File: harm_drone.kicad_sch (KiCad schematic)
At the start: 13 parts, among them IC1 Microcontroller, J1 SYS_DEBUG

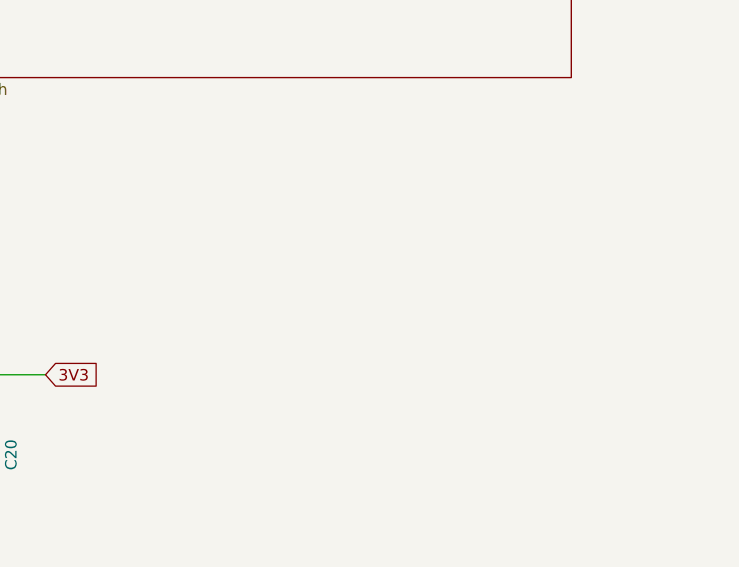
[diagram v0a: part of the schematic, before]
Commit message: before model updates
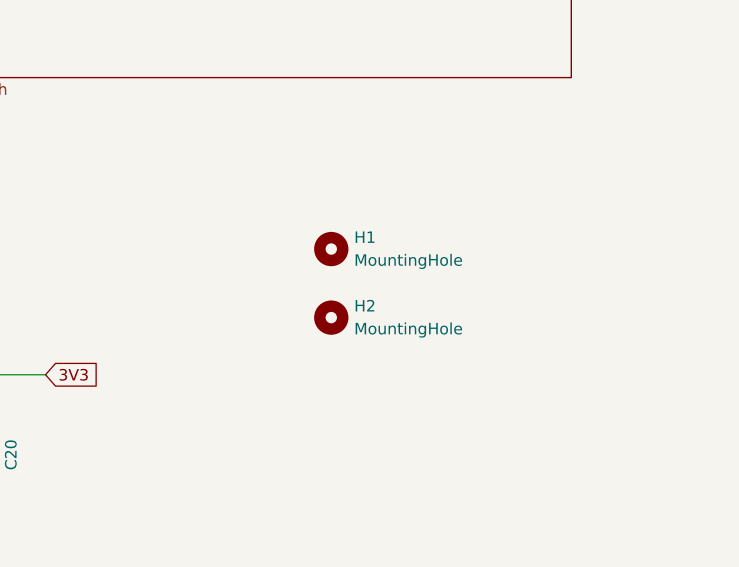
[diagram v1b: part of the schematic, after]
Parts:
- added H1, H2: MountingHole, MountingHole:MountingHole_3.2mm_M3, symbol Mechanical:MountingHole
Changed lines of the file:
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@@
+	)
+	(symbol
+		(lib_id "Mechanical:MountingHole")
+		(at 240.03 83.82 0)
+		(unit 1)
+		(exclude_from_sim yes)
+		(in_bom no)
+		(on_board yes)
+		(dnp no)
+		(fields_autoplaced yes)
+		(property "Reference" "H1"
+			(at 242.57 82.5499 0)
+			(effects
+				(font
+					(size 1.27 1.27)
+				)
+				(justify left)
+			)
+		)
+		(property "Value" "MountingHole"
+			(at 242.57 85.0899 0)
+			(effects
+				(font
+					(size 1.27 1.27)
+				)
+				(justify left)
+			)
+		)
+		(property "Footprint" "MountingHole:MountingHole_3.2mm_M3"
+			(at 240.03 83.82 0)
+			(effects
+				(font
+					(size 1.27 1.27)
+				)
+				(hide yes)
+			)
+		)
+		(property "Datasheet" "~"
+			(at 240.03 83.82 0)
+			(effects
+				(font
+					(size 1.27 1.27)
+				)
+				(hide yes)
+			)
+		)
+		(property "Description" "Mounting Hole without connection"
+			(at 240.03 83.82 0)
+			(effects
+				(font
+					(size 1.27 1.27)
+				)
+				(hide yes)
+			)
+		)
+		(instances
+			(project ""
+				(path "/5ce3566e-4e0f-420e-9b0d-3952cd3c63fd"
+					(reference "H1")
+					(unit 1)
+				)
+			)
+		)
 	)
 	(symbol
@@
 					(unit 1)
 				)
+			)
+		)
+	)
+	(symbol
+		(lib_id "Mechanical:MountingHole")
+		(at 240.03 91.44 0)
+		(unit 1)
+		(exclude_from_sim yes)
+		(in_bom no)
+		(on_board yes)
+		(dnp no)
+		(fields_autoplaced yes)
+		(property "Reference" "H2"
+			(at 242.57 90.1699 0)
+			(effects
+				(font
+					(size 1.27 1.27)
+				)
+				(justify left)
+			)
+		)
+		(property "Value" "MountingHole"
+			(at 242.57 92.7099 0)
+			(effects
+				(font
+					(size 1.27 1.27)
+				)
+				(justify left)
+			)
+		)
+		(property "Footprint" "MountingHole:MountingHole_3.2mm_M3"
+			(at 240.03 91.44 0)
+			(effects
+				(font
+					(size 1.27 1.27)
+				)
+				(hide yes)
+			)
+		)
+		(property "Datasheet" "~"
+			(at 240.03 91.44 0)
+			(effects
+				(font
+					(size 1.27 1.27)
+				)
+				(hide yes)
+			)
+		)
+		(property "Description" "Mounting Hole without connection"
+			(at 240.03 91.44 0)
+			(effects
+				(font
+					(size 1.27 1.27)
+				)
+				(hide yes)
+			)
+		)
+		(instances
+			(project "harm_drone"
+				(path "/5ce3566e-4e0f-420e-9b0d-3952cd3c63fd"
+					(reference "H2")
+					(unit 1)
+				)

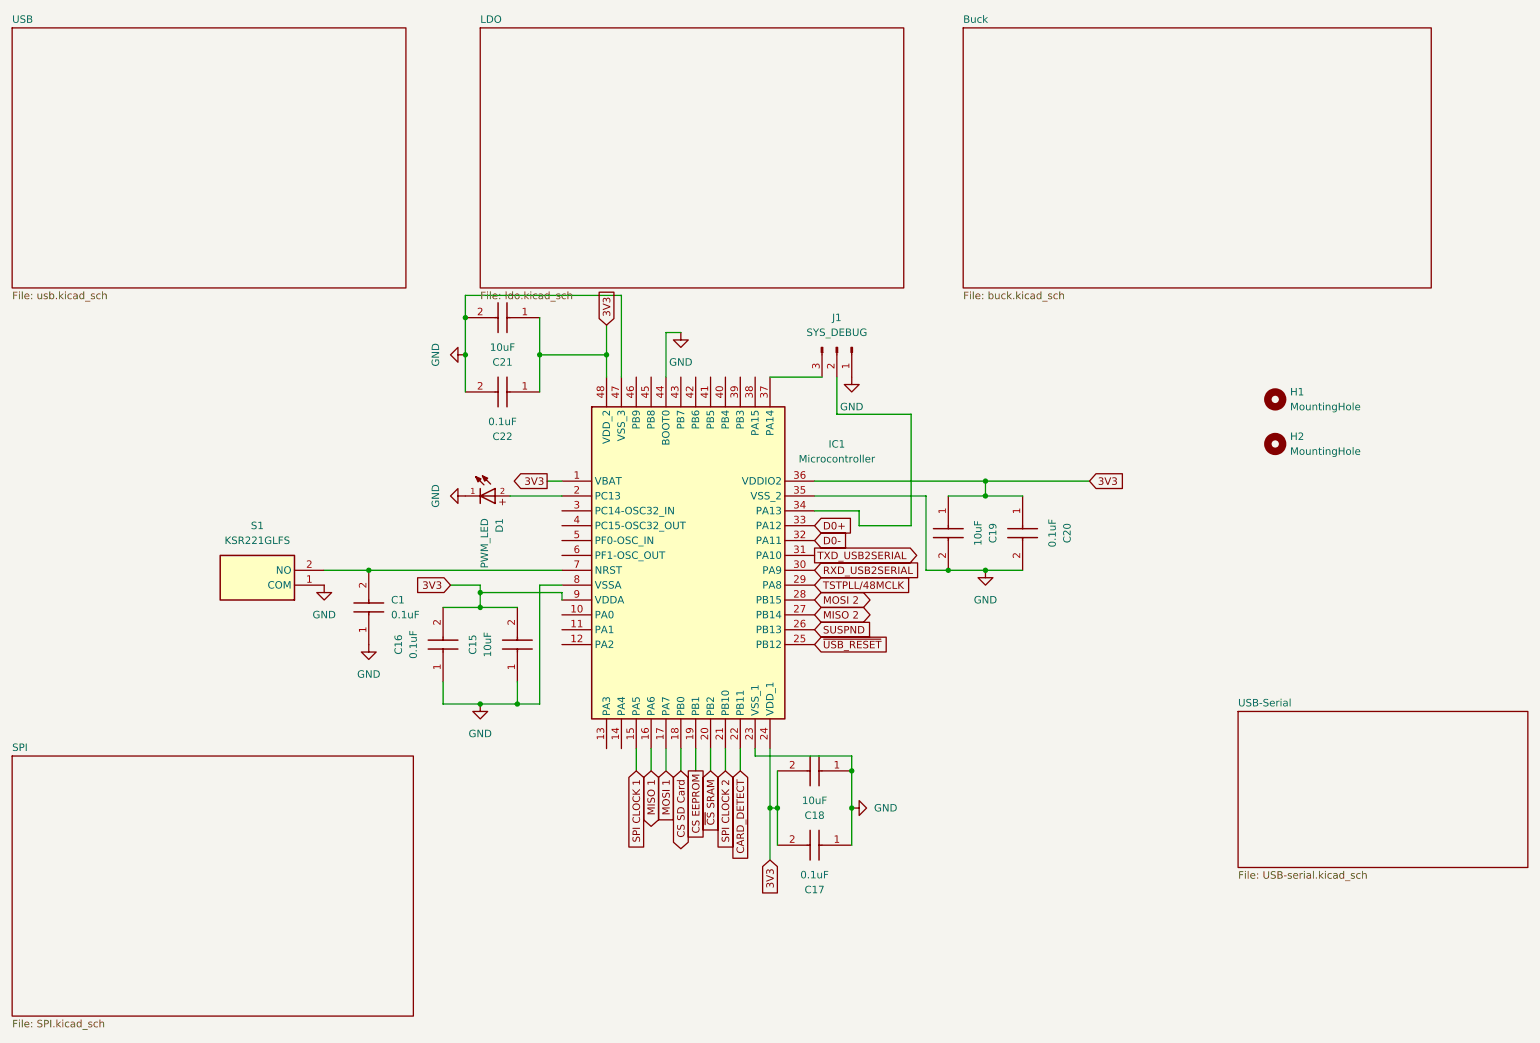
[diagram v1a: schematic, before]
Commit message: schematic fixes are done
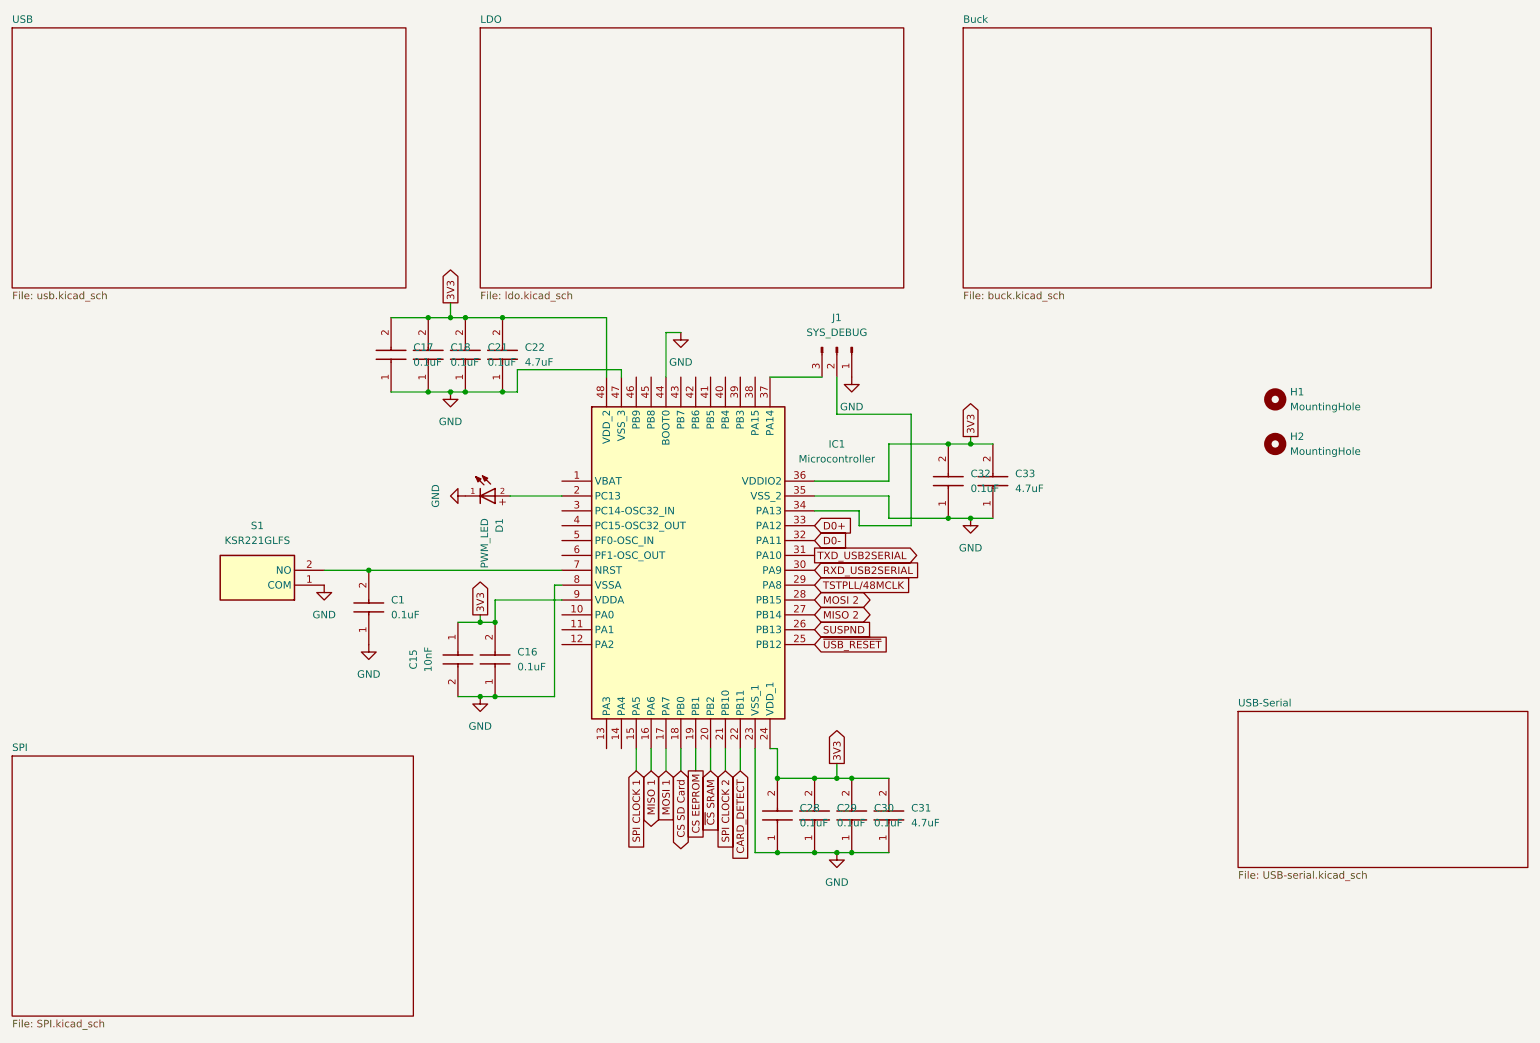
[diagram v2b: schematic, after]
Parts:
- removed C19: 10uF, Capacitor_SMD:C_0805_2012Metric, symbol group127:0805Capacitor
- removed C20: 0.1uF, Capacitor_SMD:C_0805_2012Metric, symbol group127:0805Capacitor
- added C28, C29, C30, C32: 0.1uF, Capacitor_SMD:C_0805_2012Metric, symbol group127:0805Capacitor
- added C31, C33: 4.7uF, Capacitor_SMD:C_0805_2012Metric, symbol group127:0805Capacitor
- C15: value 10uF -> 10nF
- C18, C21: value 10uF -> 0.1uF
- C22: value 0.1uF -> 4.7uF
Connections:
- net 3V3: now also C15.1, C21.2, C22.2, C28.2, C29.2, C30.2, C31.2, C32.2, C33.2; no longer C15.2, C21.1, C22.1, IC1.1 (VBAT)
- net GND: now also C15.2, C21.1, C22.1, C28.1, C29.1, C30.1, C31.1, C32.1, C33.1; no longer C15.1, C21.2, C22.2

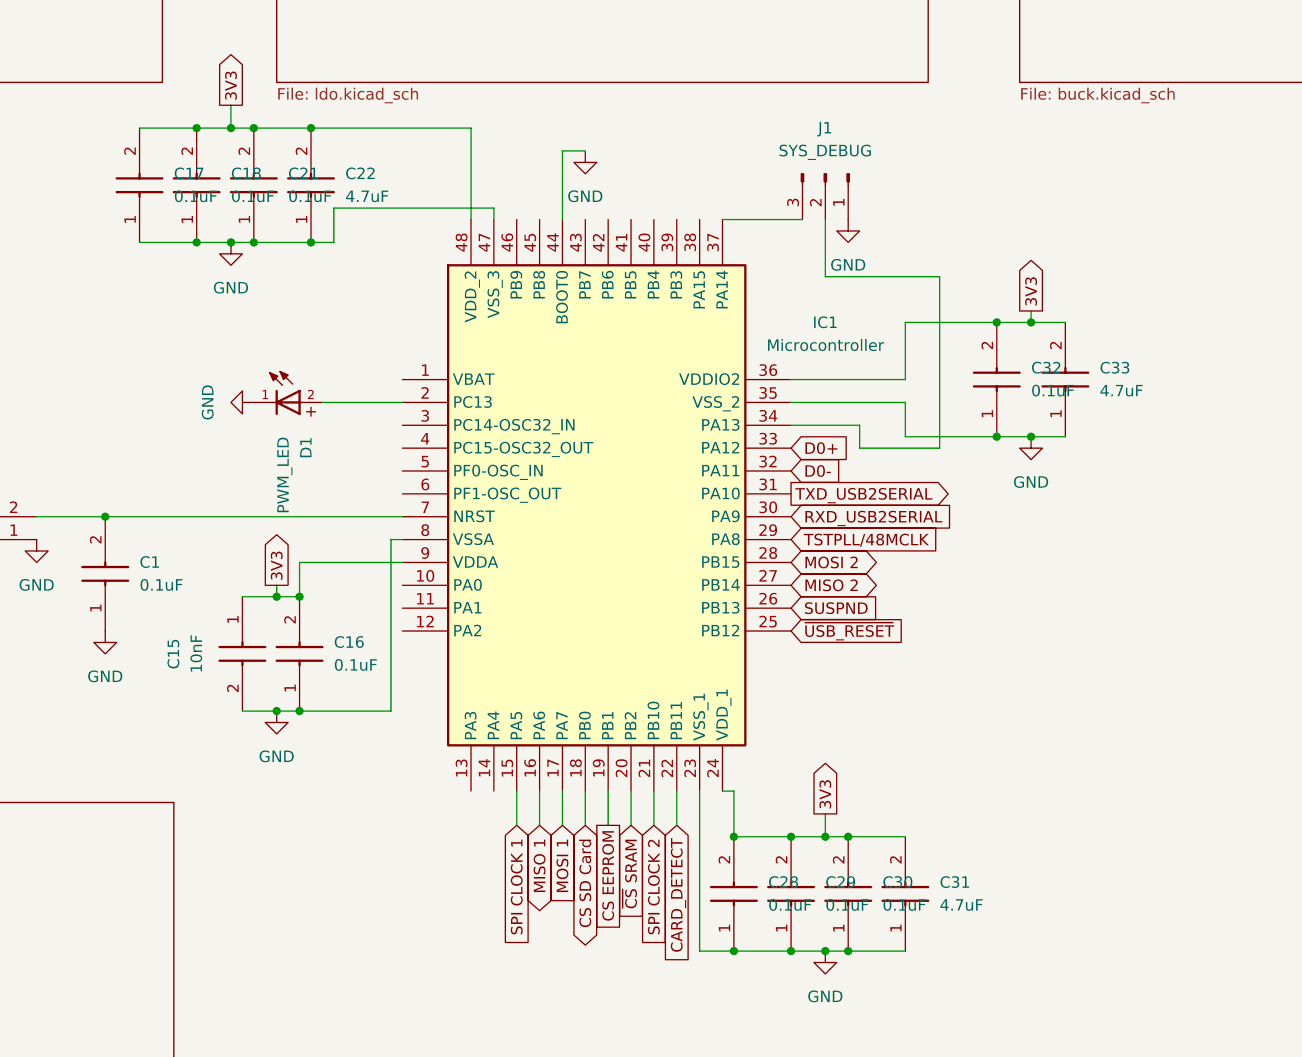
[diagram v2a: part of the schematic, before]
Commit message: final changes
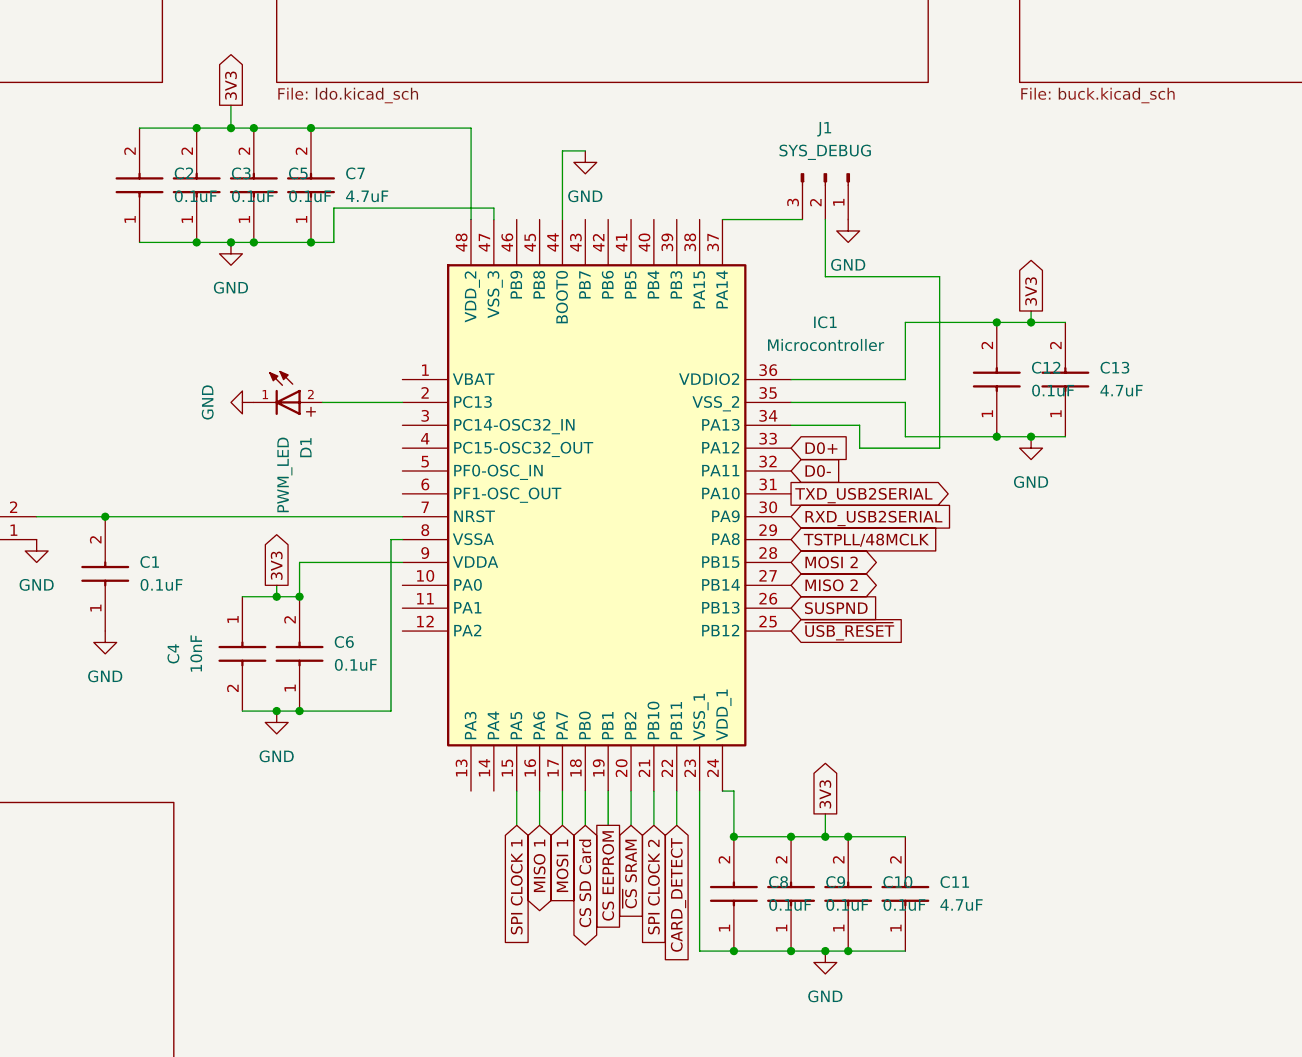
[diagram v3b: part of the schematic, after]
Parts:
- renumbered C30 to C10, C31 to C11, C32 to C12, C33 to C13, C17 to C2, C18 to C3, C15 to C4, C21 to C5, C16 to C6, C22 to C7, C28 to C8, C29 to C9
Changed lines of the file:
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@@
 		(dnp no)
 		(fields_autoplaced yes)
-		(property "Reference" "C32"
+		(property "Reference" "C12"
 			(at 187.96 96.5199 90)
 			(effects
@@
 			(project "harm_drone"
 				(path "/5ce3566e-4e0f-420e-9b0d-3952cd3c63fd"
-					(reference "C32")
+					(reference "C12")
 					(unit 1)
 				)
@@
 		(dnp no)
 		(fields_autoplaced yes)
-		(property "Reference" "C31"
+		(property "Reference" "C11"
 			(at 177.8 153.6699 90)
 			(effects
@@
 			(project "harm_drone"
 				(path "/5ce3566e-4e0f-420e-9b0d-3952cd3c63fd"
-					(reference "C31")
+					(reference "C11")
 					(unit 1)
 				)
@@
 		(dnp no)
 		(fields_autoplaced yes)
-		(property "Reference" "C33"
+		(property "Reference" "C13"
 			(at 195.58 96.5199 90)
 			(effects
@@
 			(project "harm_drone"
 				(path "/5ce3566e-4e0f-420e-9b0d-3952cd3c63fd"
-					(reference "C33")
+					(reference "C13")
 					(unit 1)
 				)
@@
 		(dnp no)
 		(fields_autoplaced yes)
-		(property "Reference" "C29"
+		(property "Reference" "C9"
 			(at 165.1 153.6699 90)
 			(effects
@@
 			(project "harm_drone"
 				(path "/5ce3566e-4e0f-420e-9b0d-3952cd3c63fd"
-					(reference "C29")
+					(reference "C9")
 					(unit 1)
 				)
@@
 		(dnp no)
 		(fields_autoplaced yes)
-		(property "Reference" "#PWR05"
+		(property "Reference" "#PWR06"
 			(at 138.43 78.74 0)
 			(effects
@@
 			(project "harm_drone"
 				(path "/5ce3566e-4e0f-420e-9b0d-3952cd3c63fd"
-					(reference "#PWR05")
+					(reference "#PWR06")
 					(unit 1)
 				)
@@
 		(dnp no)
 		(fields_autoplaced yes)
-		(property "Reference" "#PWR06"
+		(property "Reference" "#PWR05"
 			(at 104.14 140.97 0)
 			(effects
@@
 			(project "harm_drone"
 				(path "/5ce3566e-4e0f-420e-9b0d-3952cd3c63fd"
-					(reference "#PWR06")
+					(reference "#PWR05")
 					(unit 1)
 				)
@@
 		(dnp no)
 		(fields_autoplaced yes)
-		(property "Reference" "#PWR04"
+		(property "Reference" "#PWR09"
 			(at 187.96 110.49 0)
 			(effects
@@
 			(project "harm_drone"
 				(path "/5ce3566e-4e0f-420e-9b0d-3952cd3c63fd"
-					(reference "#PWR04")
+					(reference "#PWR09")
 					(unit 1)
 				)
@@
 		(dnp no)
 		(fields_autoplaced yes)
-		(property "Reference" "#PWR03"
+		(property "Reference" "#PWR07"
 			(at 165.1 167.64 0)
 			(effects
@@
 			(project "harm_drone"
 				(path "/5ce3566e-4e0f-420e-9b0d-3952cd3c63fd"
-					(reference "#PWR03")
+					(reference "#PWR07")
 					(unit 1)
 				)
@@
 		(dnp no)
 		(fields_autoplaced yes)
-		(property "Reference" "#PWR021"
+		(property "Reference" "#PWR04"
 			(at 95.25 100.33 0)
 			(effects
@@
 			(project "harm_drone"
 				(path "/5ce3566e-4e0f-420e-9b0d-3952cd3c63fd"
-					(reference "#PWR021")
+					(reference "#PWR04")
 					(unit 1)
 				)
@@
 		(dnp no)
 		(fields_autoplaced yes)
-		(property "Reference" "C18"
+		(property "Reference" "C3"
 			(at 99.06 74.9299 90)
 			(effects
@@
 			(project "harm_drone"
 				(path "/5ce3566e-4e0f-420e-9b0d-3952cd3c63fd"
-					(reference "C18")
+					(reference "C3")
 					(unit 1)
 				)
@@
 		(dnp no)
 		(fields_autoplaced yes)
-		(property "Reference" "C30"
+		(property "Reference" "C10"
 			(at 171.45 153.6699 90)
 			(effects
@@
 			(project "harm_drone"
 				(path "/5ce3566e-4e0f-420e-9b0d-3952cd3c63fd"
-					(reference "C30")
+					(reference "C10")
 					(unit 1)
 				)
@@
 		(on_board yes)
 		(dnp no)
-		(property "Reference" "C15"
+		(property "Reference" "C4"
 			(at 92.71 128.27 0)
 			(effects
@@
 			(project "harm_drone"
 				(path "/5ce3566e-4e0f-420e-9b0d-3952cd3c63fd"
-					(reference "C15")
+					(reference "C4")
 					(unit 1)
 				)
@@
 		(dnp no)
 		(fields_autoplaced yes)
-		(property "Reference" "C16"
+		(property "Reference" "C6"
 			(at 110.49 126.9999 90)
 			(effects
@@
 			(project "harm_drone"
 				(path "/5ce3566e-4e0f-420e-9b0d-3952cd3c63fd"
-					(reference "C16")
+					(reference "C6")
 					(unit 1)
 				)
@@
 		(dnp no)
 		(fields_autoplaced yes)
-		(property "Reference" "C22"
+		(property "Reference" "C7"
 			(at 111.76 74.9299 90)
 			(effects
@@
 			(project "harm_drone"
 				(path "/5ce3566e-4e0f-420e-9b0d-3952cd3c63fd"
-					(reference "C22")
+					(reference "C7")
 					(unit 1)
 				)
@@
 		(on_board yes)
 		(dnp no)
-		(property "Reference" "C28"
+		(property "Reference" "C8"
 			(at 158.75 153.6699 90)
 			(effects
@@
 			(project "harm_drone"
 				(path "/5ce3566e-4e0f-420e-9b0d-3952cd3c63fd"
-					(reference "C28")
+					(reference "C8")
 					(unit 1)
 				)
@@
 		(on_board yes)
 		(dnp no)
-		(property "Reference" "C17"
+		(property "Reference" "C2"
 			(at 92.71 74.9299 90)
 			(effects
@@
 			(project "harm_drone"
 				(path "/5ce3566e-4e0f-420e-9b0d-3952cd3c63fd"
-					(reference "C17")
+					(reference "C2")
 					(unit 1)
 				)
@@
 		(dnp no)
 		(fields_autoplaced yes)
-		(property "Reference" "#PWR08"
+		(property "Reference" "#PWR03"
 			(at 99.06 88.9 0)
 			(effects
@@
 			(project "harm_drone"
 				(path "/5ce3566e-4e0f-420e-9b0d-3952cd3c63fd"
-					(reference "#PWR08")
+					(reference "#PWR03")
 					(unit 1)
 				)
@@
 		(dnp no)
 		(fields_autoplaced yes)
-		(property "Reference" "C21"
+		(property "Reference" "C5"
 			(at 105.41 74.9299 90)
 			(effects
@@
 			(project "harm_drone"
 				(path "/5ce3566e-4e0f-420e-9b0d-3952cd3c63fd"
-					(reference "C21")
+					(reference "C5")
 					(unit 1)
 				)
@@
 		(dnp no)
 		(fields_autoplaced yes)
-		(property "Reference" "#PWR07"
+		(property "Reference" "#PWR08"
 			(at 167.64 86.36 0)
 			(effects
@@
 			(project "harm_drone"
 				(path "/5ce3566e-4e0f-420e-9b0d-3952cd3c63fd"
-					(reference "#PWR07")
+					(reference "#PWR08")
 					(unit 1)
 				)
